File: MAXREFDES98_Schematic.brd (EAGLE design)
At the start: 87.8 x 25.4 mm, 34 parts, among them U1 MB110S-TP, U2 MB110S-TP, U3 MAX5969AETB+

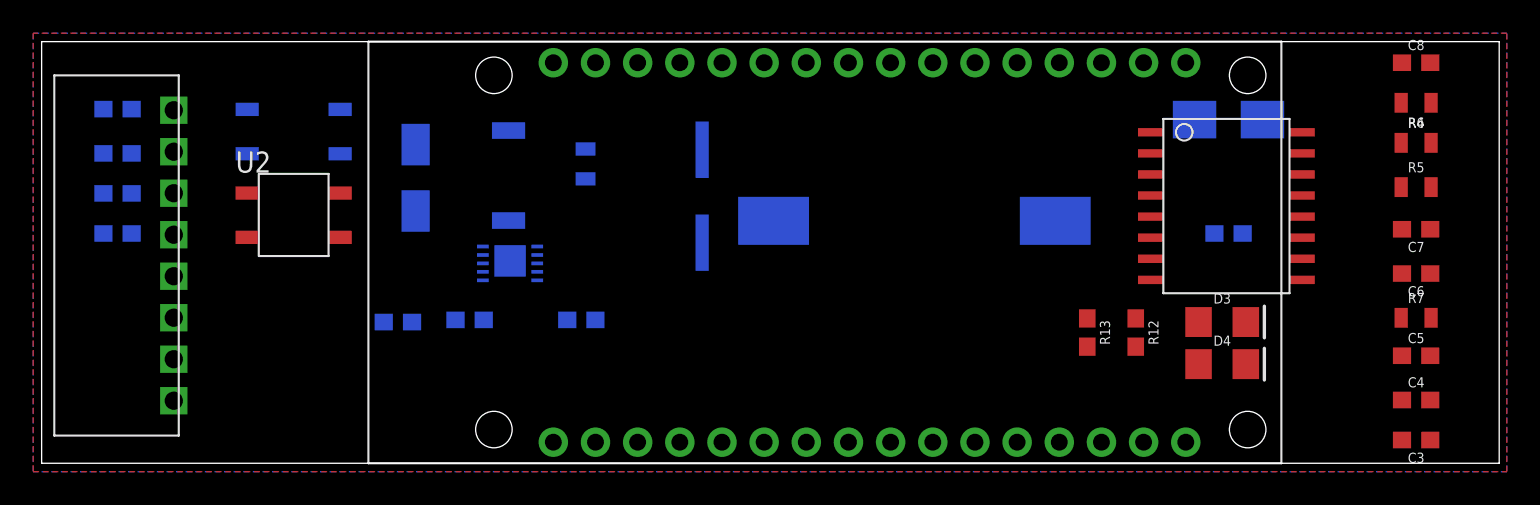
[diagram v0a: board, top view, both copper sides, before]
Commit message: Update MAXREFDES98_Schematic.brd
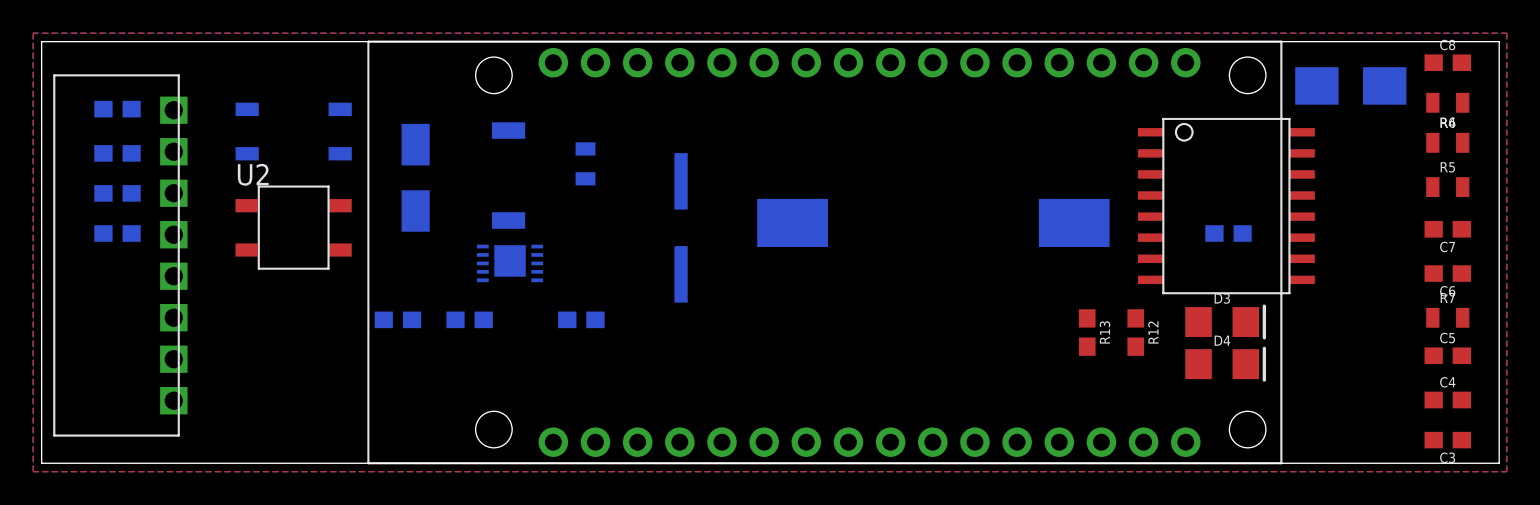
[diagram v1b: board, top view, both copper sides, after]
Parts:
- moved D2 7.64 mm to (78.9, 22.7)
- moved C2 2.29 mm to (42.7, 10.0)
- moved C3 1.91 mm to (84.7, 1.40)
- moved C4 1.91 mm to (84.7, 3.81)
- moved C5 1.91 mm to (84.7, 6.48)
- moved C6 1.91 mm to (84.7, 11.4)
- moved C7 1.91 mm to (84.7, 14.1)
- moved C8 1.91 mm to (84.7, 24.1)
- moved R4 1.91 mm to (84.7, 19.3)
- moved R5 1.91 mm to (84.7, 16.6)
- moved R6 1.91 mm to (84.7, 21.7)
- moved R7 1.91 mm to (84.7, 8.76)
- moved L2_150UH 1.15 mm to (53.7, 14.5)
- moved U2 0.76 mm to (11.7, 12.4)
- moved R1 0.13 mm to (21.5, 8.64)
